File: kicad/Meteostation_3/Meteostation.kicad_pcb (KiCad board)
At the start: 2 copper layers, 45 x 45 mm, 94 parts, among them J1 TxD, J12 TxD_AirS8, J13 RxD_AirS8, J14 +5v, J2 RxD, J3 BME280_SCL, J4 BME280_SDA, J5 RST, J6 +EXT, J7 -EXT, J8 RxD_AirS8(D8), J9 TxD_AirS8(D9), Q1 5N10, T1 HY931147C, U1 ATmega328P-AU, U6 NCP1117-3.3, Y1 Crystal_GND2, Y2 ECS-250-20-33

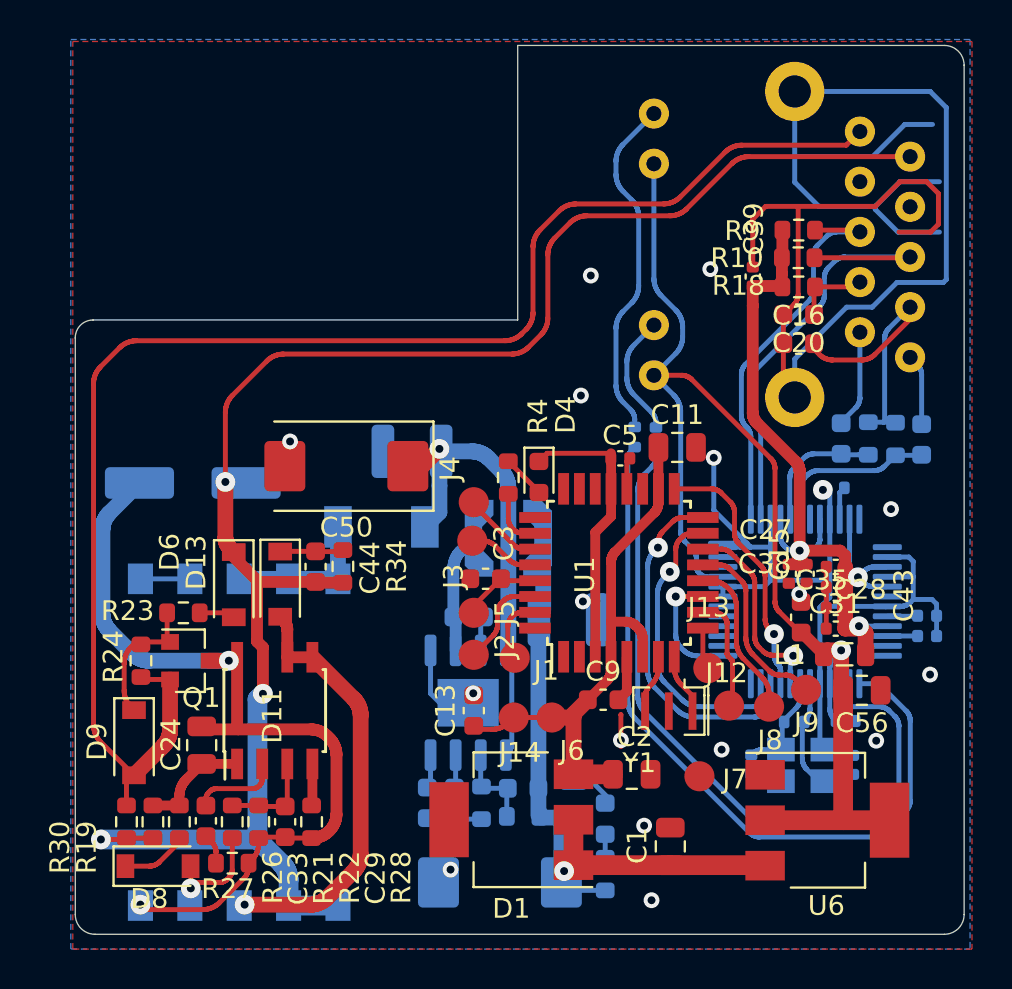
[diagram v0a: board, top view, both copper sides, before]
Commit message: изменено:      kicad/Meteostation_3/Meteostation.kicad_pcb 	изменено:      kicad/Meteostation_3/Meteostation.kicad_pcb-bak 	изменено:      kicad/Meteostation_3/Meteostation.sch 	изменено:      kicad/Meteostation_3/Meteostation.sch-bak 	изменено:      kicad/Meteostation_3/gerber/Border.gbr 	изменено:      kicad/Meteostation_3/gerber/Bottom.gbr 	изменено:      kicad/Meteostation_3/gerber/MaskBottom.gbr 	изменено:      kicad/Meteostation_3/gerber/MaskTop.gbr 	изменено:      kicad/Meteostation_3/gerber/Meteostation-job.gbrjob 	изменено:      kicad/Meteostation_3/gerber/Meteostation.zip 	изменено:      kicad/Meteostation_3/gerber/NCData.drl 	изменено:      kicad/Meteostation_3/gerber/Top.gbr
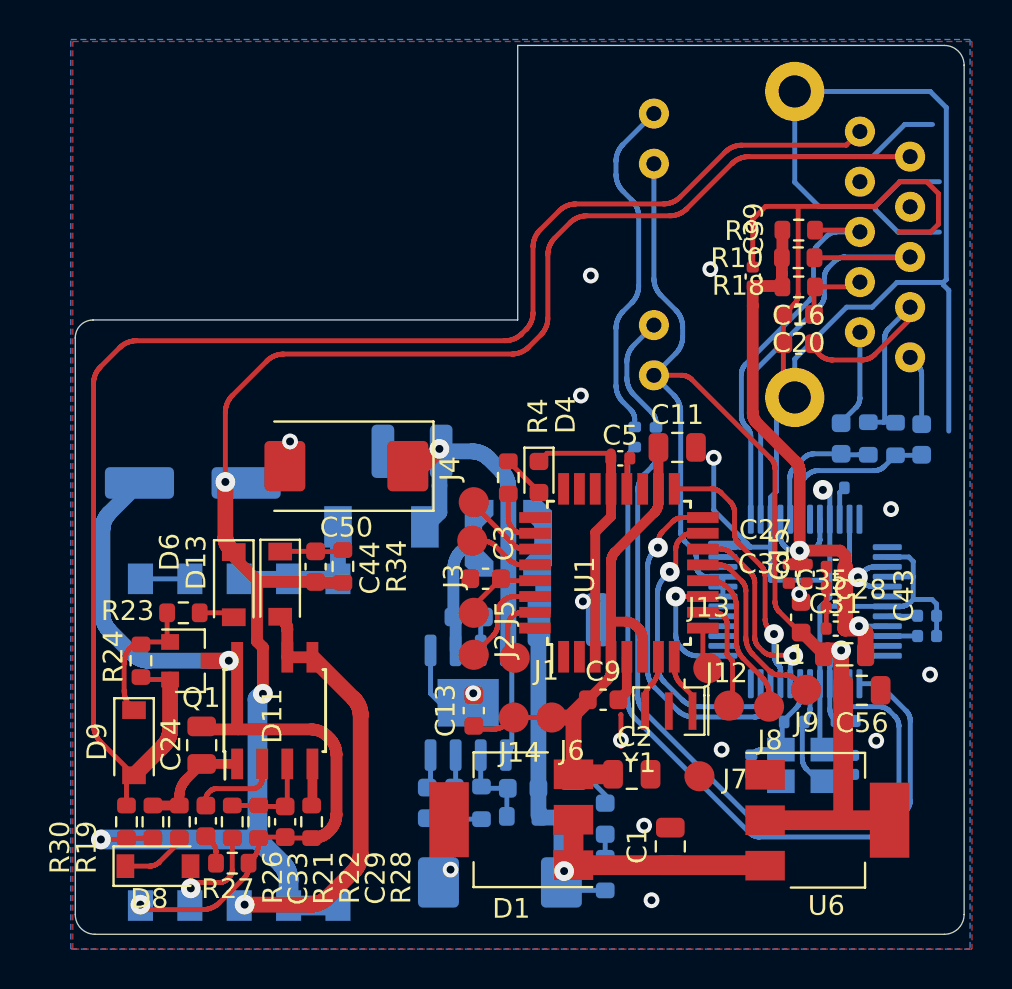
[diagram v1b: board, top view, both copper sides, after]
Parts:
- Y1: value Crystal_GND2 -> 16MHz
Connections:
- D3 pad 43: GND -> +3.3VDAC
- D3 pad 44: GND -> +3.3VDAC
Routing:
- net GND: track 164.0 -> 175.3 mm
- net +3.3VDAC: track 62.3 -> 63.3 mm
